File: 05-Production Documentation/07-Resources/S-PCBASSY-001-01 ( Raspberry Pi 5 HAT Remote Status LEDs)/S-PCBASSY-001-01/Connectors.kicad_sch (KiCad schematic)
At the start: 18 parts, among them Q1 BSS138, Q2 BSS138, Q3 BSS138

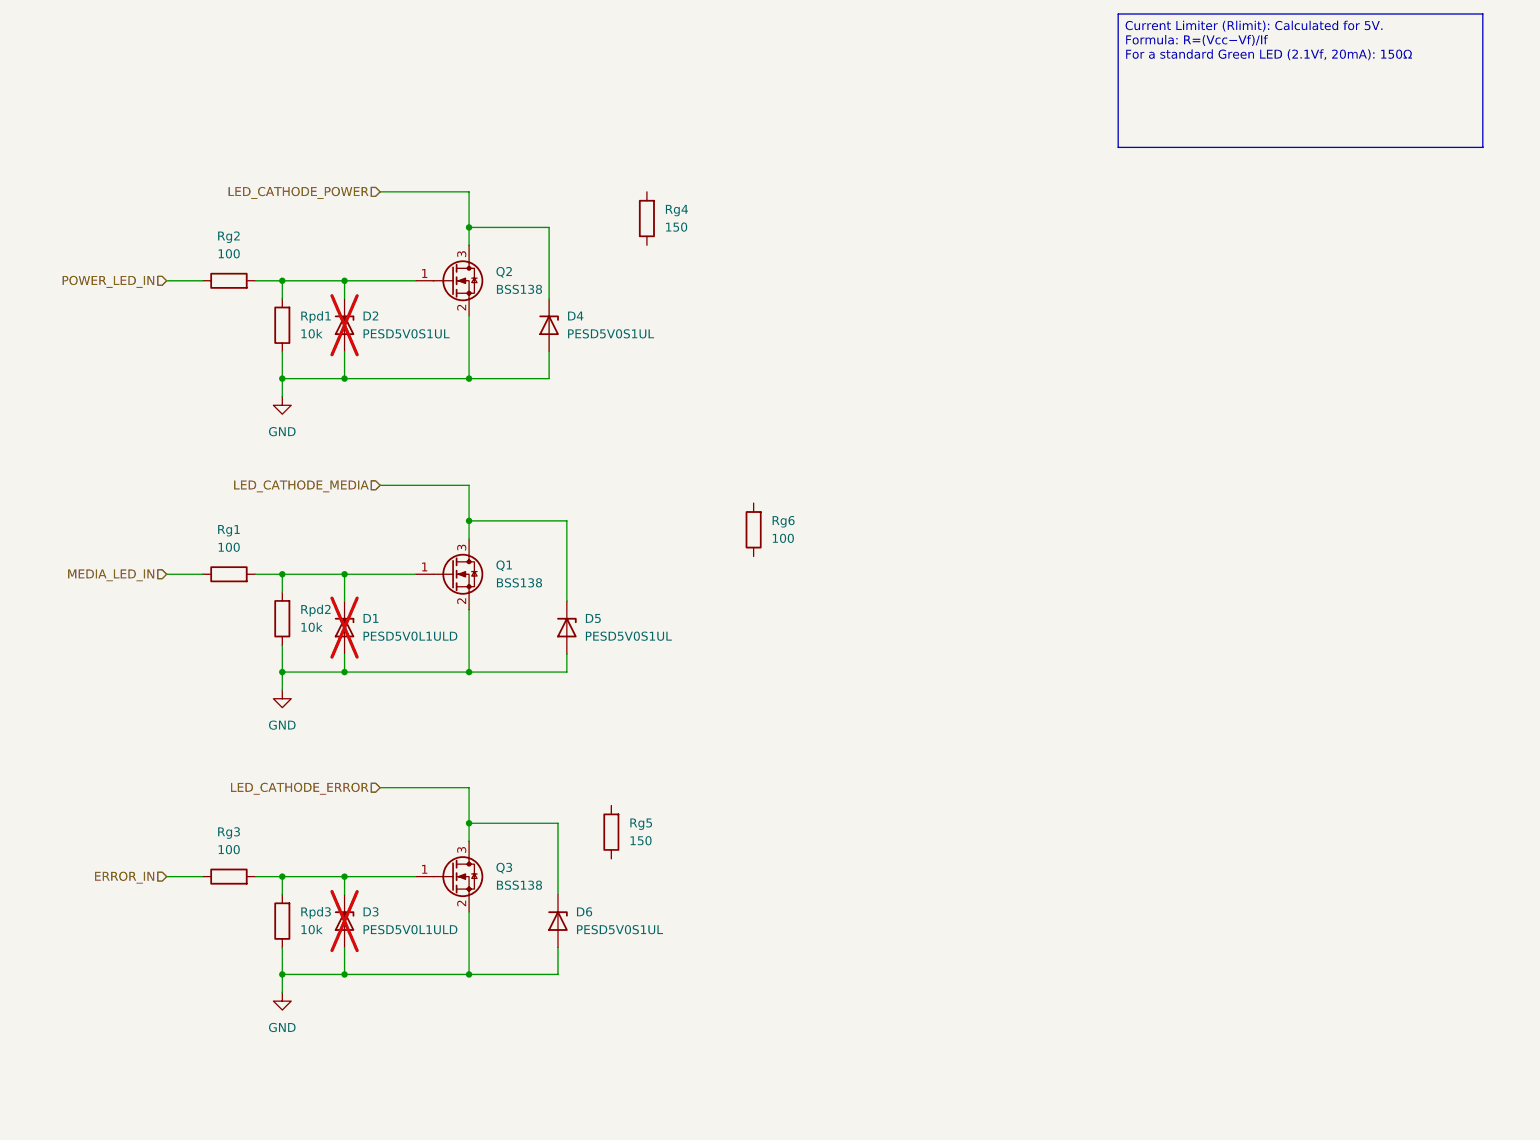
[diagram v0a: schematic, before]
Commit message: WIP - LED Driver and Started with Connectors
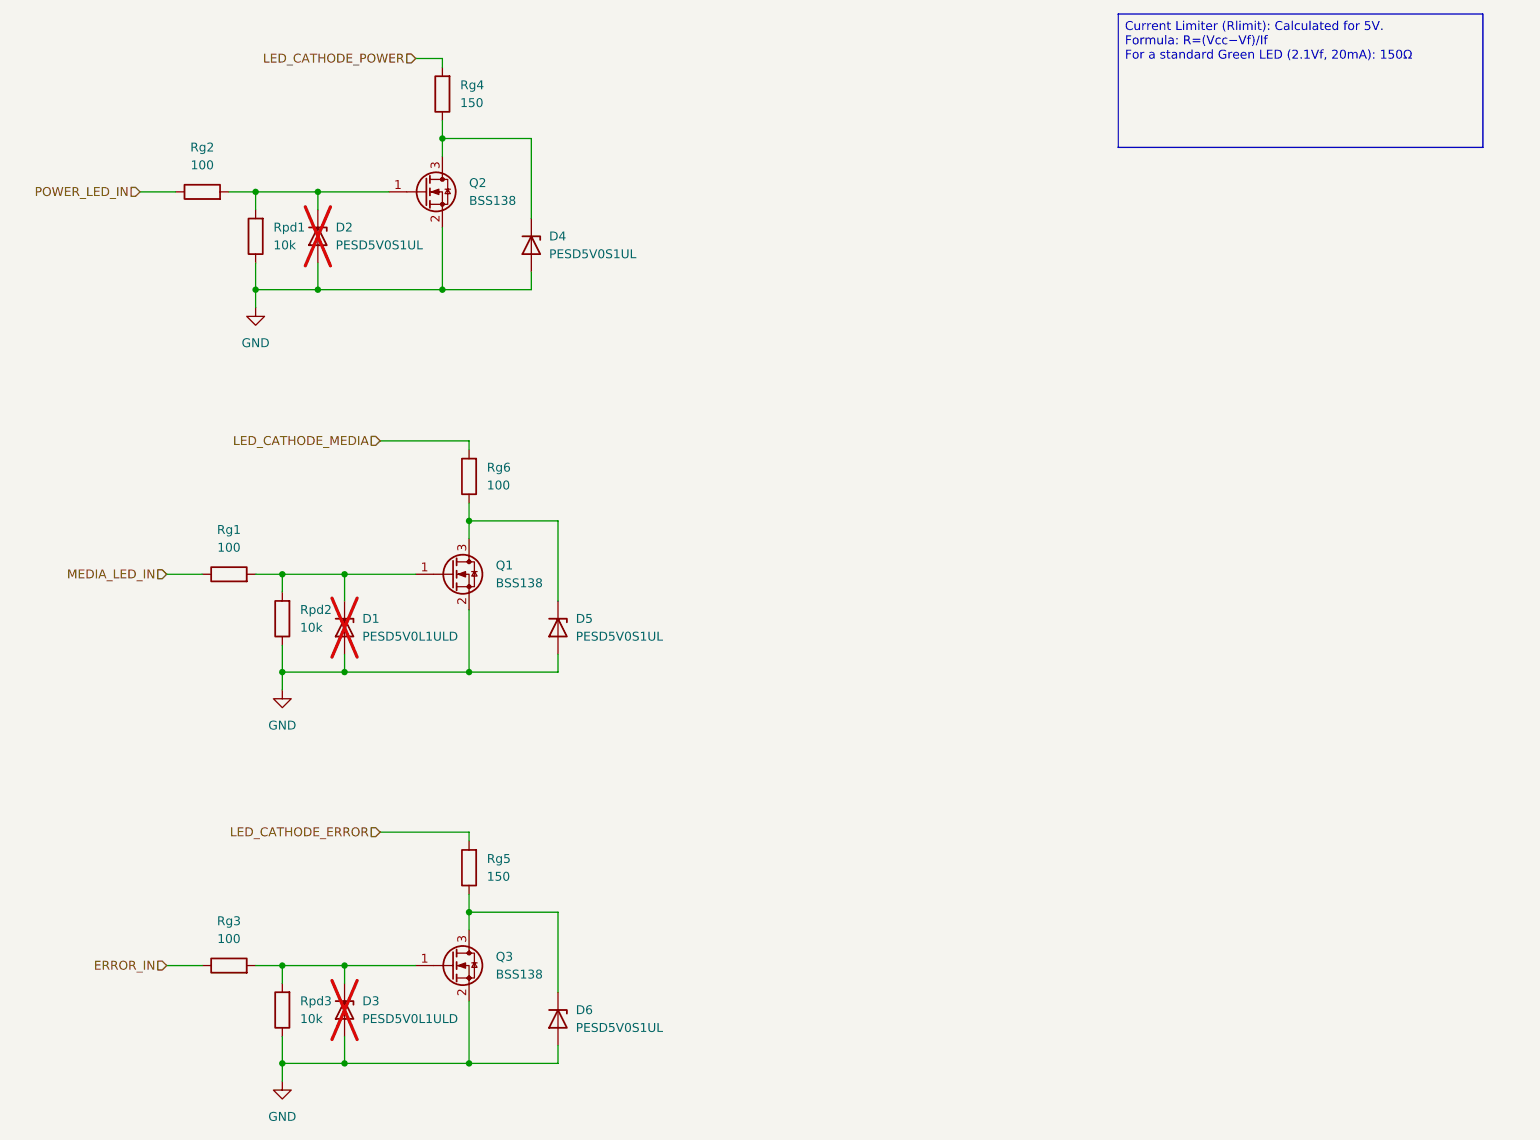
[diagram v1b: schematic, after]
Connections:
- net LED_CATHODE_ERROR: now also Rg5.2; no longer D6.1 (K), Q3.3 (D)
- net LED_CATHODE_MEDIA: now also Rg6.2; no longer D5.1 (K), Q1.3 (D)
- net LED_CATHODE_POWER: now also Rg4.2; no longer D4.1 (K), Q2.3 (D)
- net at Rg4.1: now also D4.1 (K), Q2.3 (D)
- net at Rg5.1: now also D6.1 (K), Q3.3 (D)
- net at Rg6.1: now also D5.1 (K), Q1.3 (D)
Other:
- moved on the sheet: D2, D3, D4, D5, D6, Q2, Q3, Rg2, Rg3, Rg4, Rg5, Rg6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
